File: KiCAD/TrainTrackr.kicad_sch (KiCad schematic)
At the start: 0 parts

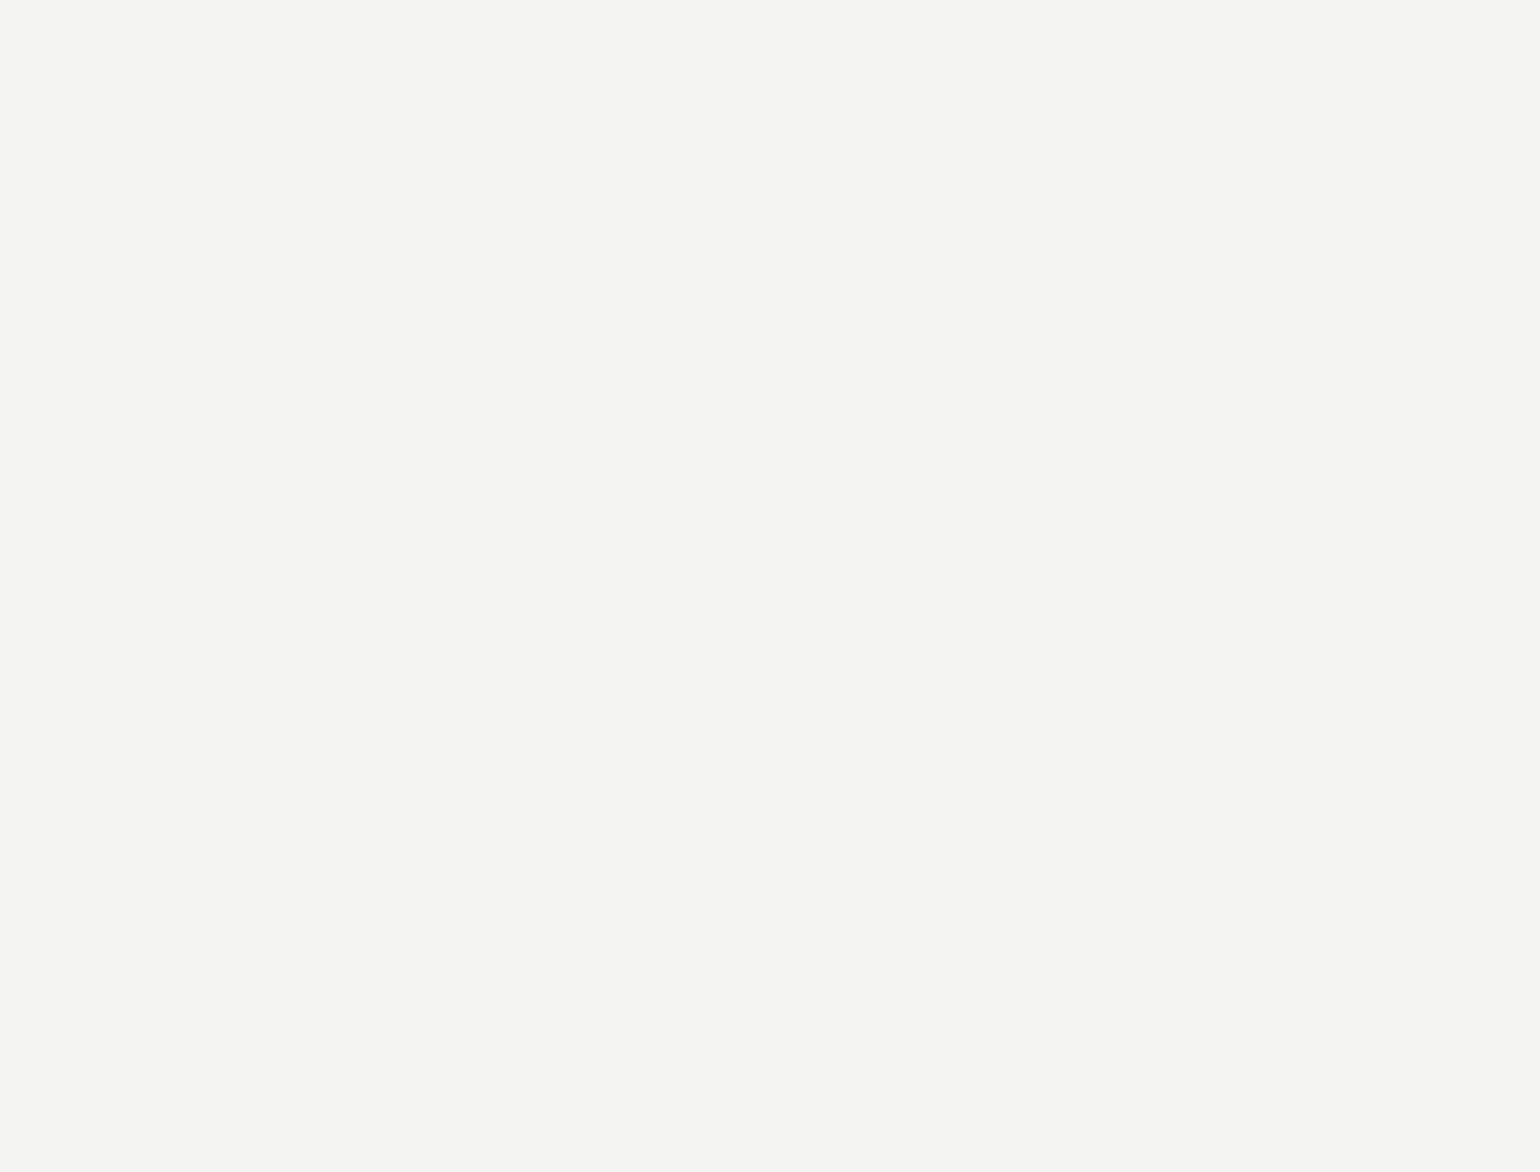
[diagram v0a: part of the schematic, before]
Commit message: updated sch
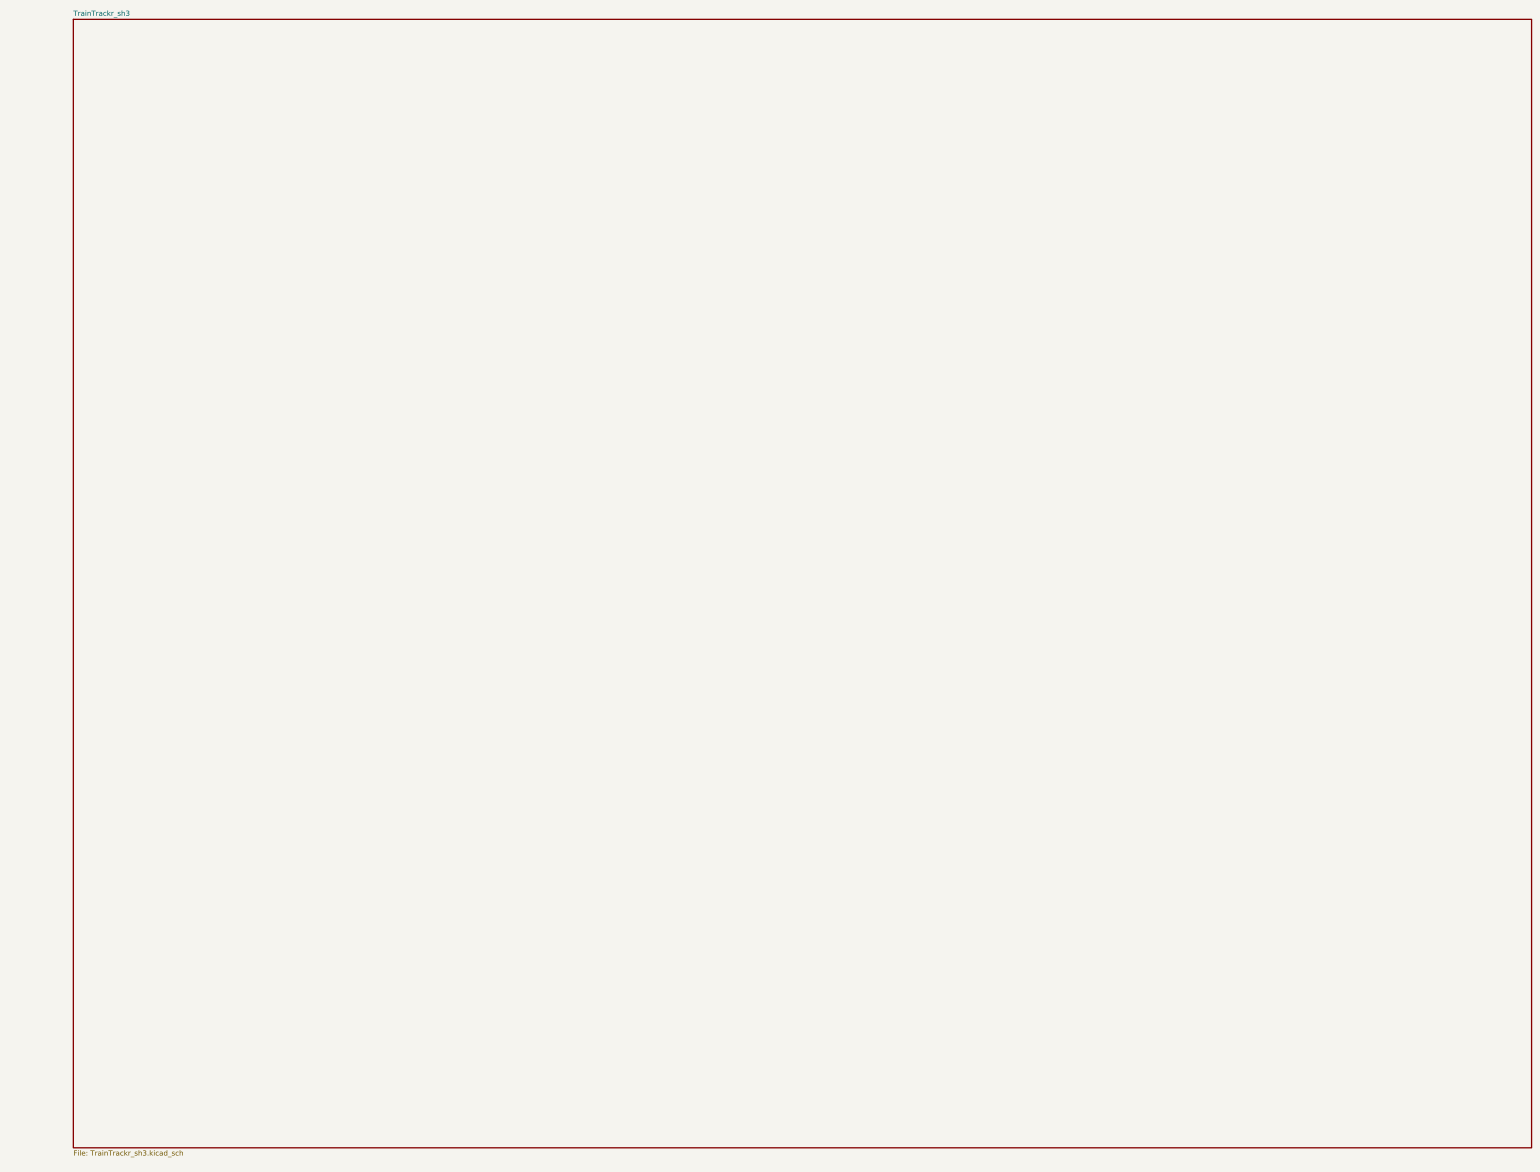
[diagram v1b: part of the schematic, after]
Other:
- added sheet TrainTrackr_sh3 (TrainTrackr_sh3.kicad_sch)
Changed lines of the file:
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@@
+		)
+	)
+	(sheet
+		(at 852.17 0)
+		(size 359.41 278.13)
+		(fields_autoplaced yes)
+		(stroke
+			(width 0.1524)
+			(type solid)
+		)
+		(fill
+			(color 0 0 0 0.0000)
+		)
+		(property "Sheetname" "TrainTrackr_sh3"
+			(at 852.17 -0.7116 0)
+			(effects
+				(font
+					(size 1.27 1.27)
+				)
+				(justify left bottom)
+			)
+		)
+		(property "Sheetfile" "TrainTrackr_sh3.kicad_sch"
+			(at 852.17 278.7146 0)
+			(effects
+				(font
+					(size 1.27 1.27)
+				)
+				(justify left top)
+			)
+		)
+		(instances
+			(project "TrainTrackr"
+				(path "/779c311e-6596-48d7-a471-956474340a54"
+					(page "3")
+				)
+			)
 		)
 	)

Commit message: updated sch
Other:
- added sheet TrainTrackr_sh4 (TrainTrackr_sh4.kicad_sch)
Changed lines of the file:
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@@
+	)
+	(sheet
+		(at -6.35 312.42)
+		(size 438.15 278.13)
+		(fields_autoplaced yes)
+		(stroke
+			(width 0.1524)
+			(type solid)
+		)
+		(fill
+			(color 0 0 0 0.0000)
+		)
+		(property "Sheetname" "TrainTrackr_sh4"
+			(at -6.35 311.7084 0)
+			(effects
+				(font
+					(size 1.27 1.27)
+				)
+				(justify left bottom)
+			)
+		)
+		(property "Sheetfile" "TrainTrackr_sh4.kicad_sch"
+			(at -6.35 591.1346 0)
+			(effects
+				(font
+					(size 1.27 1.27)
+				)
+				(justify left top)
+			)
+		)
+		(instances
+			(project "TrainTrackr"
+				(path "/779c311e-6596-48d7-a471-956474340a54"
+					(page "4")
+				)
+			)
+		)
 	)
 	(sheet
